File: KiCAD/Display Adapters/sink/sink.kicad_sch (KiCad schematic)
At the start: 7 parts, among them J1 47272-0001, J2 XT30PW_2_2_-M.G.B, J3 20455-040E-76

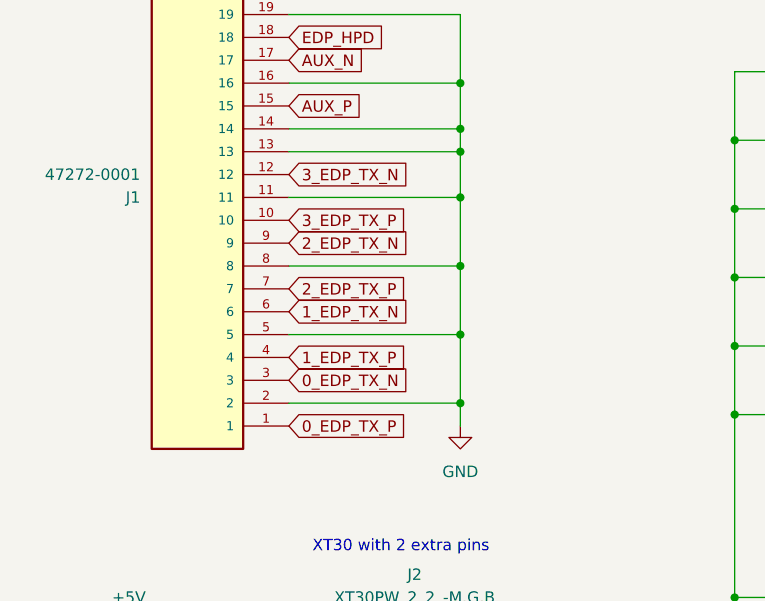
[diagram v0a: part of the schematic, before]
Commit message: updates
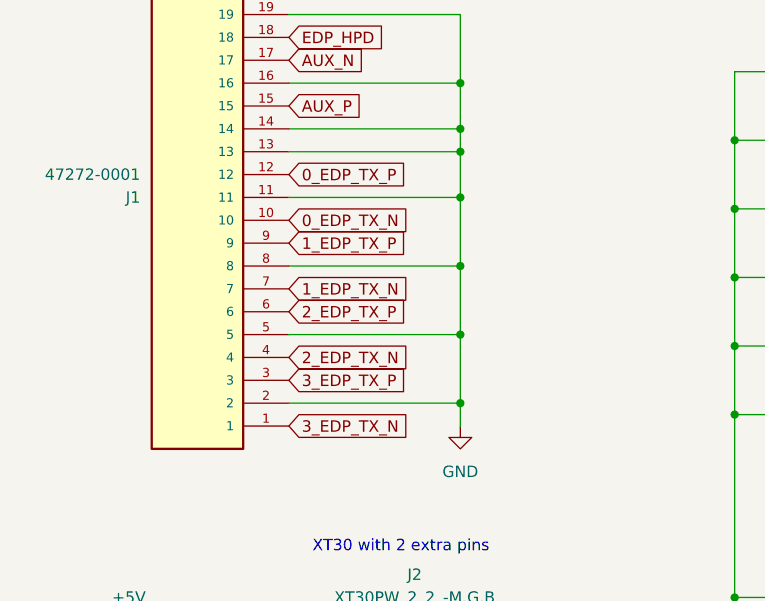
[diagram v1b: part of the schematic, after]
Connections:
- net 0_EDP_TX_N: now also J1.10; no longer J1.3
- net 0_EDP_TX_P: now also J1.12; no longer J1.1
- net 1_EDP_TX_N: now also J1.7; no longer J1.6
- net 1_EDP_TX_P: now also J1.9; no longer J1.4
- net 2_EDP_TX_N: now also J1.4; no longer J1.9
- net 2_EDP_TX_P: now also J1.6; no longer J1.7
- net 3_EDP_TX_N: now also J1.1; no longer J1.12
- net 3_EDP_TX_P: now also J1.3; no longer J1.10

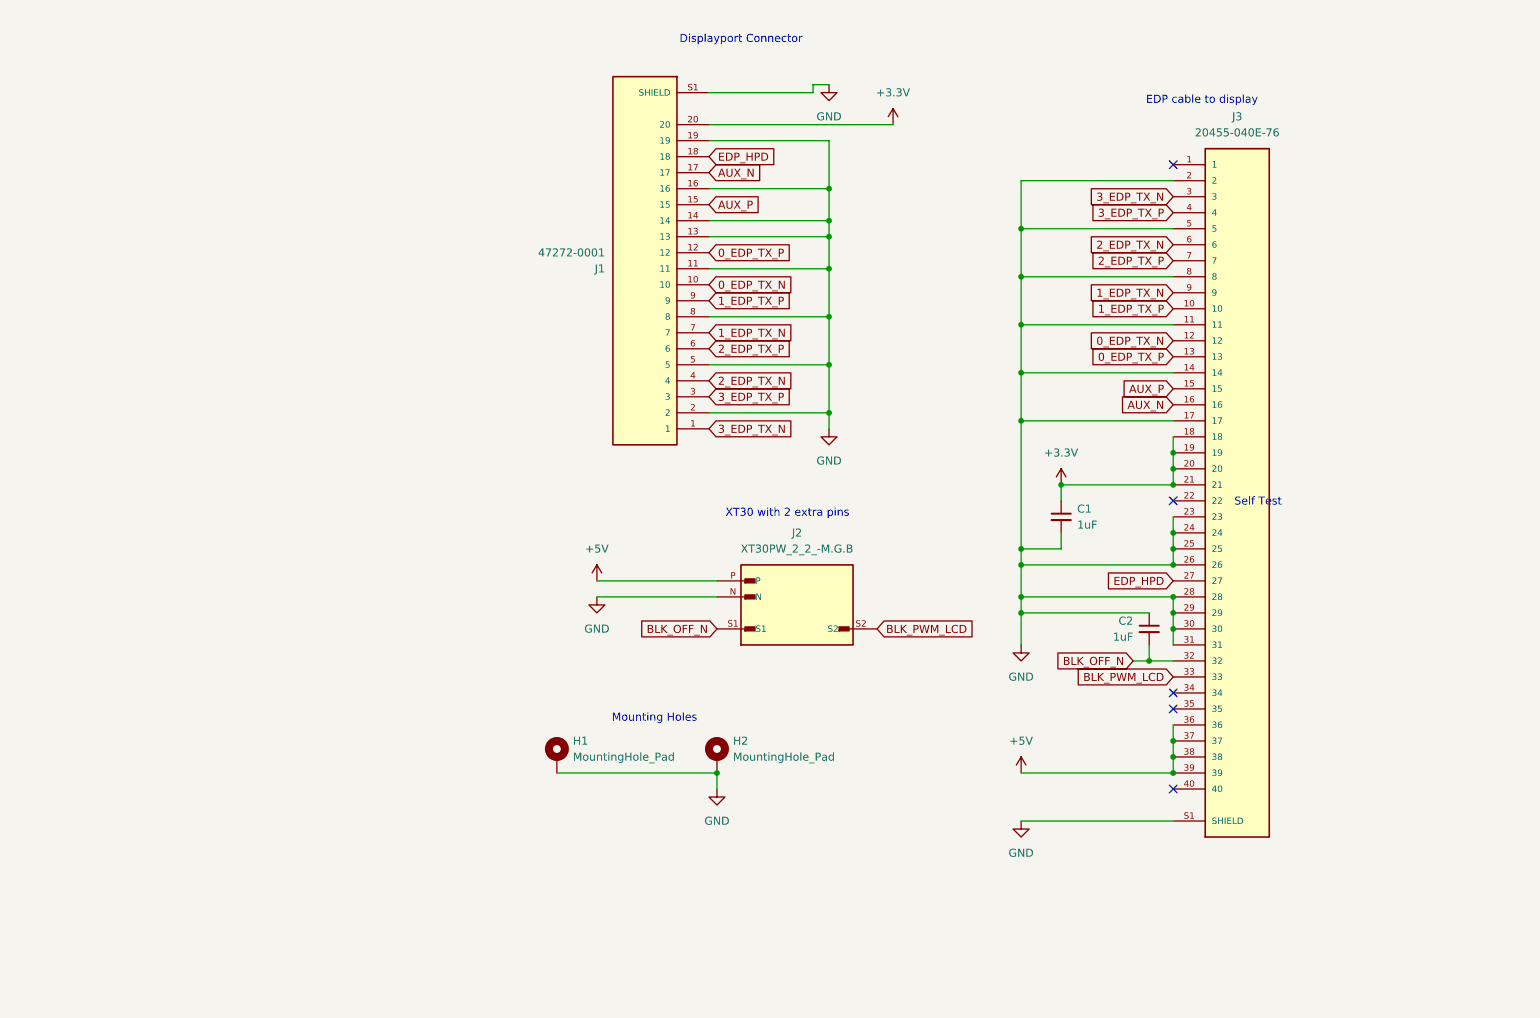
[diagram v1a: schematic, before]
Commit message: fix schematics
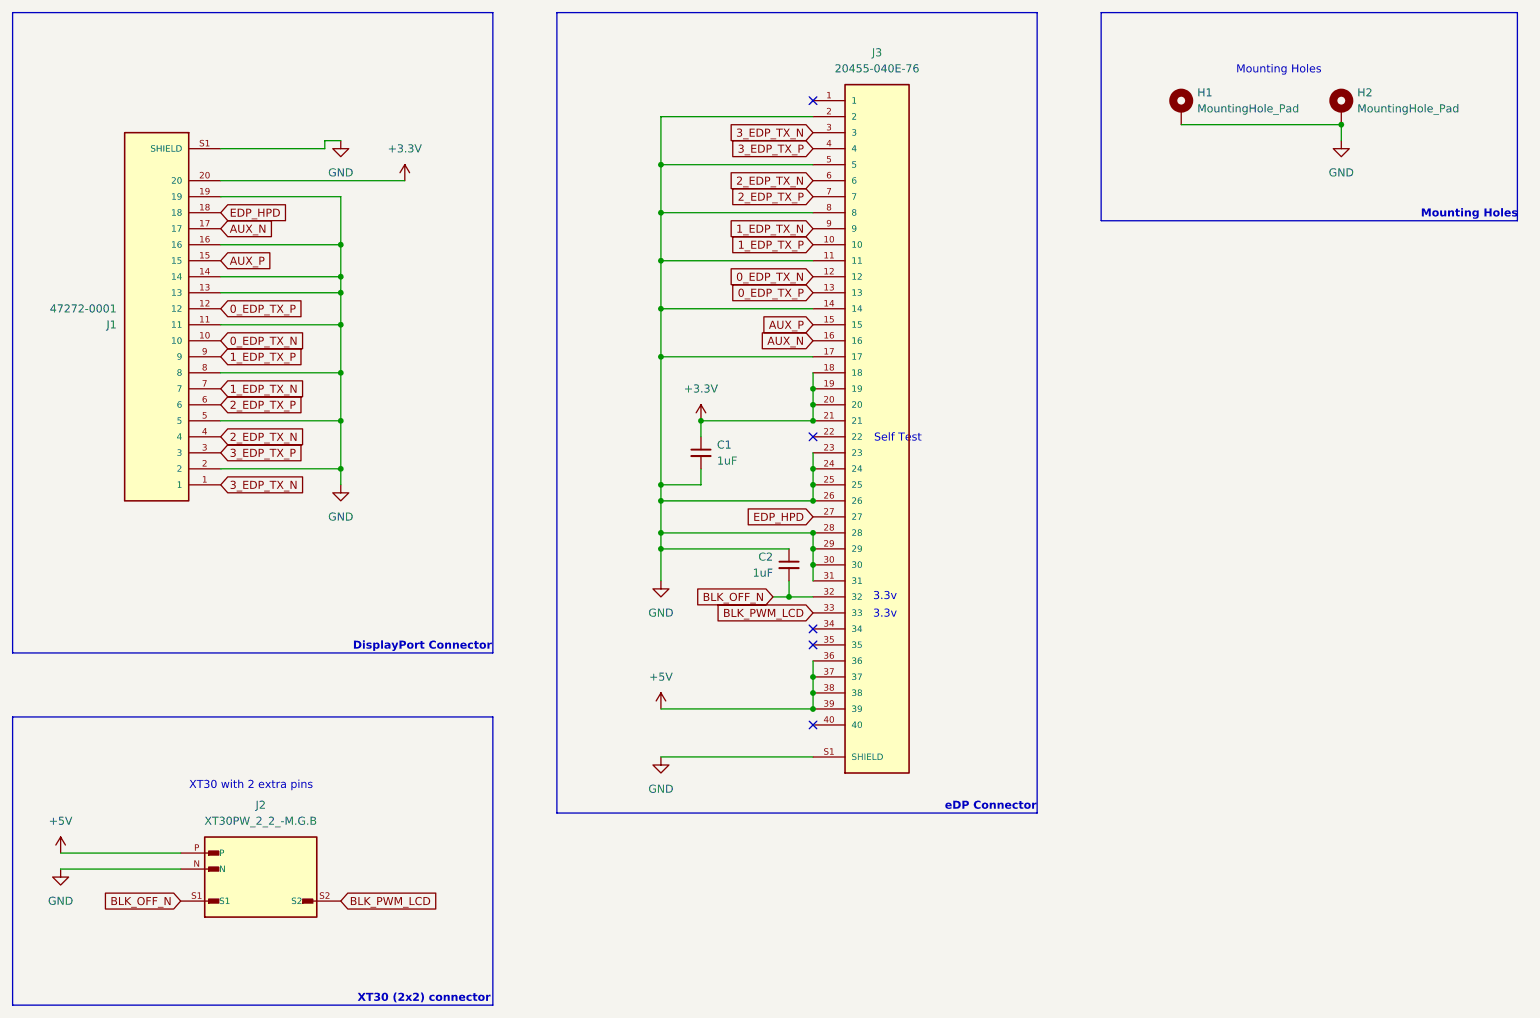
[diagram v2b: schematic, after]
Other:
- note added: "3.3v"
- note added: "DisplayPort Connector"
- note added: "XT30 (2x2) connector"
- note added: "eDP Connector"
- note removed: "Displayport Connector"
- note removed: "EDP cable to display"
- title: (none) -> Sink: DP to eDP
- moved on the sheet: C1, C2, H1, H2, J1, J2, J3
